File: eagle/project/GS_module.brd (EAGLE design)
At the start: 101.3 x 81.3 mm, 103 parts, among them IC1 LM358, Q2 MOSFET-PCHANNELFQP27P06, U1 V_REG_317SMD

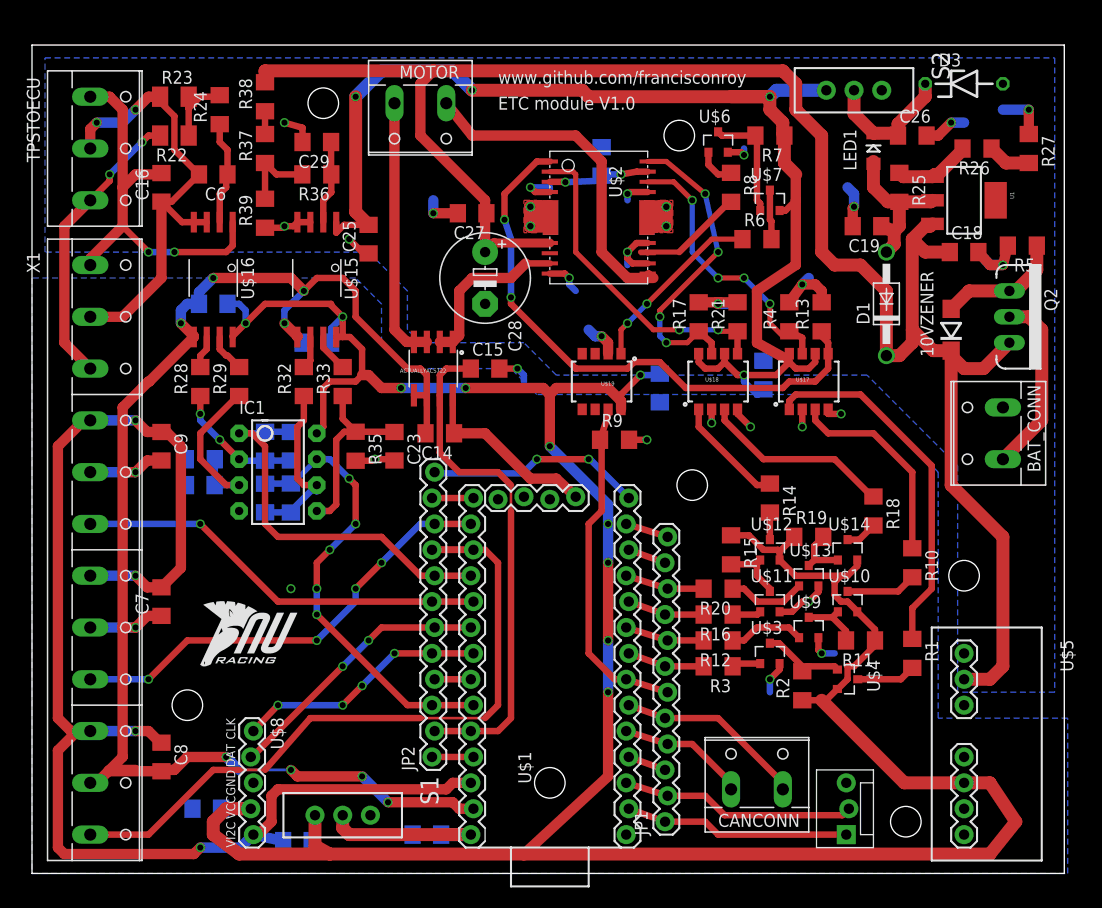
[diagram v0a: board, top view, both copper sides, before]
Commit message: finish version 1.0 of GS board
yay!
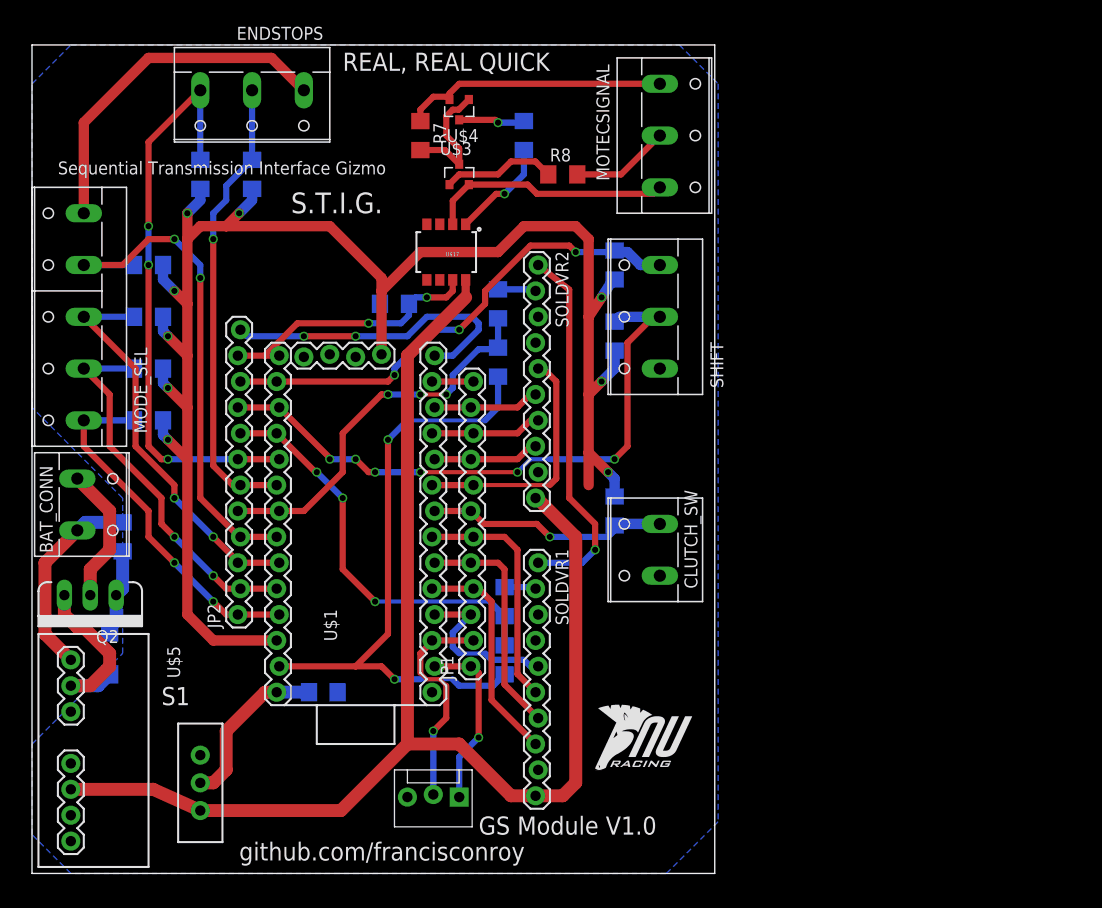
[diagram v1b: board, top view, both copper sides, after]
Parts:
- removed ACTUALLYACS722: ACS722, SparkFun-AnalogIC:SO08
- removed C10, C14, C8: 0.1 uF, rcl:C1206
- removed C13, C26, C3: 0.1uF, resistor:C1206
- removed C15, C20, C21, C22, C23: 1nF, rcl:C1206
- removed C16, C17, C18, C24, C25, C4, C5, C7, C9: 0.1uF, rcl:C1206
- removed C19, C27: 1uF, rcl:C1206
- removed C28: 47uF, rcl:E5-8,5
- removed C29, C6: 10n, rcl:C1206
- removed CANCONN, MOTOR: (no value), con-wago-508:W237-132
- removed D1: 1N4004, diode:DO41-10
- removed D3: 7.5V, diode:ZDIO-7.5
- removed IC1: LM358, SparkFun-AnalogIC:DIP08
- removed LED1: FUSE HERE, LilyPad-Wearables:LED-1206
- removed R19: 10k, resistor:R1206
- removed R20: 4.7k, resistor:R1206
- removed R21: 1k, resistor:R1206
- removed R22: 3k, rcl:M1206
- removed R23: 2k, rcl:M1206
- removed R24, R36: 39, rcl:R1206
- removed R25: 240, rcl:R1206
- removed R26: 680, rcl:R1206
- removed R27: 33, rcl:R1206
- removed R28, R29, R31, R32, R33, R35: 20k, rcl:R1206
- removed R30, R34: 40k, rcl:R1206
- removed R37: 56k, rcl:R1206
- removed R38: 4k7, rcl:R1206
- removed R39: 9k1, rcl:R1206
- removed S2: DIRTY 5V, SparkFun-Electromechanical:SWITCH-SPDT_KIT
- removed TPSTOECU: (no value), con-wago-508:W237-133
- removed U$10, U$12, U$14, U$7: PNP_TRAN, custom:SOT23-3
- removed U$11, U$13, U$6, U$9: NPN_TRAN, custom:SOT23-3
- removed U$15, U$16: ACPLC87BT, custom:SO8STRETCH
- removed U$18, U$19: OPTOISOLATOR-2SOIC8, SparkFun-DiscreteSemi:SO08-2
- removed U$20: (no value), custom:NURLOGO
- removed U$8: DISP_CONN, custom:DISP_CONN
- removed U1: V_REG_317SMD, SparkFun-PowerIC:SOT223
- removed X1: (no value), con-wago-508:W237-12P
- added CLUTCH_SW: (no value), con-wago-508:W237-132
- added ENDSTOPS, MOTECSIGNAL, SHIFT: (no value), con-wago-508:W237-133
- added MODE_SEL: (no value), con-wago-508:W237-5P
- added SOLDVR1, SOLDVR2: (no value), SparkFun-Connectors:1X10_LOCK
- R1: value 270 -> 27; device resistor:R1206 -> rcl:R1206
- R10, R14, R18: value 270 -> 10k; device resistor:R1206 -> rcl:R1206
- R11, R15: device resistor:R1206 -> rcl:R1206
- R12, R16: value 4.7k -> 10k; device resistor:R1206 -> rcl:R1206
- R13, R17: value 1k -> 10k; device resistor:R1206 -> rcl:R1206
- R2: value 10k -> 27; device resistor:R1206 -> rcl:R1206
- R3: value 4.7k -> 15; device resistor:R1206 -> rcl:R1206
- R4: value 1k -> 15; device resistor:R1206 -> rcl:R1206
- U$2: value TB6559FG -> (none); device custom:HSOP16-P-300-1.00 -> custom:NURLOGO
- moved Q2 94.2 mm to (5.71, 27.3), turned to 180 degrees
- moved R5 92.8 mm to (8.89, 33.0), flipped to the bottom, turned to 90 degrees
- moved BAT_CONN 89.8 mm to (5.08, 36.2), turned to 270 degrees
- moved 10VZENER 88.4 mm to (7.62, 21.6), flipped to the bottom
- moved U$5 87.6 mm to (3.81, 12.1)
- moved R12 68.3 mm to (16.5, 68.6), flipped to the bottom, turned to 270 degrees
- moved U$4 67.6 mm to (41.9, 74.9), turned to 180 degrees
- moved R14 65.1 mm to (11.4, 59.7), flipped to the bottom, turned to 180 degrees
- moved R15 61.6 mm to (11.4, 54.6), flipped to the bottom, turned to 180 degrees
- moved R16 60.9 mm to (11.4, 49.5), flipped to the bottom
- moved U$2 59.9 mm to (55.2, 10.2), turned to 0 degrees
- moved R13 57.6 mm to (21.6, 68.6), flipped to the bottom, turned to 270 degrees
- moved U$3 56.0 mm to (41.9, 68.6)
- moved R17 54.9 mm to (11.4, 44.5), flipped to the bottom, turned to 180 degrees
- moved R2 43.6 mm to (45.7, 50.2), flipped to the bottom
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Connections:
- removed net +5V/1: C13.1, C25.2, R7.1, S2.3, U$15.1, U$17.6, U$17.8, U$18.6, U$18.8, U$7.2
- removed net +5VCLEAN: C17.2, C24.2, C3.1, C4.2, IC1.8, R11.1, R15.1, R19.1, R2.1, S1.3, U$10.2, U$12.2, U$14.2, U$15.8, U$16.8, U$19.8, U$4.2, U$5.6, U$8.4
- removed net 5VOUT: C10.2, U$2.VREF, U$2.VREG
- removed net ECU5V: C16.2, TPSTOECU.1, U$16.1, X1.1
- removed net ECUSENSGND: C16.1, C6.2, R23.1, TPSTOECU.2, U$16.3, U$16.4, X1.2
- removed net ECUTPS: R22.2, TPSTOECU.3, X1.3
- removed net N$11: R8.1, U$6.1
- removed net N$12: R19.2, U$13.3, U$14.1
- removed net N$14: R18.1, U$18.3
- removed net N$15: C26.1, D3.C, LED1.C, S2.2
- removed net N$16: R37.2, R38.1
- removed net N$17: C19.1, D1.A, LED1.A, R25.2, U1.2
- removed net N$18: R11.2, U$10.1, U$9.3
- removed net N$19: MOTOR.1, U$2.OUT2
- removed net N$20: ACTUALLYACS722.1, ACTUALLYACS722.2, U$2.OUT1
- removed net N$21: R10.1, U$17.3
- removed net N$22: R10.2, U$10.3
- removed net N$23: R12.1, U$9.1
- removed net N$25: R15.2, U$11.3, U$12.1
- removed net N$26: R14.1, U$18.1
- removed net N$27: R14.2, U$12.3
- removed net N$28: R16.1, U$11.1
- removed net N$29: R17.1, U$18.7, U$2.IN2
- removed net N$30: R18.2, U$14.3
- removed net N$31: R20.1, U$13.1
- removed net N$32: R8.2, U$2.ALERT
- removed net N$33: R21.1, U$18.5, U$2.SB
- removed net N$34: ACTUALLYACS722.3, ACTUALLYACS722.4, MOTOR.2
- removed net N$35: C6.1, R24.1, U$16.2
- removed net N$36: R22.1, R23.2, R24.2
- removed net N$37: R26.1, R27.2
- removed net N$38: R25.1, R26.2, U1.1
- removed net N$39: R36.2, R37.1, R39.2
- removed net N$40: C23.1, IC1.5, R33.1, R35.1
- removed net N$41: C22.2, IC1.6, R32.1, R34.2
- removed net N$42: R32.2, U$15.6
- removed net N$43: R13.1, U$17.5, U$2.IN1
- removed net N$44: R29.2, U$16.7
- removed net N$45: C21.1, IC1.3, R29.1, R31.1
- removed net N$46: C20.2, IC1.2, R28.1, R30.2
- removed net N$47: R28.2, U$16.6
- removed net N$48: C29.1, R36.1, U$15.2
- removed net N$52: R33.2, U$15.7
- new net +5V: S1.3, SOLDVR1.10, SOLDVR2.10, U$17.8, U$5.6
- new net +5V/4: MOTECSIGNAL.1, R7.1, U$4.2
- new net GND4: MOTECSIGNAL.3, U$17.2, U$3.2
- net +12V: no longer C18.1, C27.1, C28.+, D1.C, R38.2, U$2.VCC, U1.3
- net +3V3: now also R10.2, R11.2, R12.2, R13.2, R14.2, R15.2, R16.2, R17.2, R18.2; no longer ACTUALLYACS722.8, C14.1, C5.2, C7.2, C8.1, C9.1, U$8.5, X1.10, X1.4, X1.7
- net AGND: now also R1.1, R2.1; no longer ACTUALLYACS722.5, ACTUALLYACS722.6, C14.2, C17.1, C24.1, C7.1, C8.2, C9.2, U$15.5, U$16.5, X1.11, X1.5, X1.8
- net GND: now also CLUTCH_SW.1, ENDSTOPS.1, MODE_SEL.5, SHIFT.1, SOLDVR1.9, SOLDVR2.9; no longer C15.2, C21.2, C23.2, C3.2, C4.1, C5.1, IC1.4, R31.2, R35.2, U$11.2, U$13.2, U$17.2, U$17.4, U$18.2, U$18.4, U$3.2, U$8.3, U$9.2
- net GNDI: no longer C10.1, C13.2, C18.2, C19.2, C25.1, C26.2, C27.2, C28.-, C29.2, D3.A, R13.2, R17.2, R21.2, R27.1, R39.1, R4.2, S2.1, U$15.3, U$15.4, U$19.2, U$2.FIN, U$2.FIN2, U$2.P$20, U$2.P$4, U$2.P-GND, U$2.RSA, U$2.S-GND, U$2.S-GND2, U$2.S-GND3, U$6.2
- net N$1: now also R7.2; no longer R2.2
- net N$10: now also SOLDVR1.1, SOLDVR2.1; no longer R6.2, U$7.3
- net N$3: now also R3.2, SOLDVR1.2; no longer R1.1, U$17.1
- net N$4: now also R6.1, U$17.1; no longer R1.2, U$4.3
- net N$5: now also R4.2, SOLDVR2.2; no longer R3.1, U$3.1
- net N$6: now also R6.2, U$4.3; no longer R7.2, U$6.3, U$7.1
- net N$8: now also R8.1, U$3.1; no longer R4.1, U$17.7, U$2.PWM
- net N$9: now also MOTECSIGNAL.2, R8.2; no longer R6.1, U$19.1
- net P10: now also SOLDVR2.6
- net P13: now also R9.1, U$17.7
- net P14: now also R10.1, SHIFT.3; no longer X1.9
- net P15: now also R11.1, SHIFT.2; no longer X1.12
- net P16: now also R1.2, R3.1; no longer C20.1, IC1.1, R30.1
- net P17: now also ENDSTOPS.3, R12.1; no longer X1.6
- net P18: now also ENDSTOPS.2, R13.1; no longer U$8.2
- net P19: now also R2.2, R4.1; no longer U$8.1
- net P2: now also SOLDVR1.5
- net P20: now also MODE_SEL.4, R14.1
- net P21: now also MODE_SEL.3, R15.1; no longer C22.1, IC1.7, R34.1
- net P22: now also MODE_SEL.2, R16.1; no longer ACTUALLYACS722.7, C15.1
- net P23: now also MODE_SEL.1, R17.1
- net P3: now also SOLDVR1.8; no longer CANCONN.1
- net P4: now also SOLDVR1.7; no longer CANCONN.2
- net P5: now also SOLDVR1.6; no longer R9.1, U$19.7
- net P6: now also CLUTCH_SW.2, R18.1; no longer R3.2
- net P7: now also SOLDVR2.5; no longer R12.2
- net P8: now also SOLDVR2.8; no longer R16.2
- net P9: now also SOLDVR2.7; no longer R20.2
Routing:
- net +5VCLEAN: track 276.3 -> 0.00 mm, vias 10 -> 0
- net +12V: track 183.3 -> 18.1 mm
- net +5V: track 0.00 -> 132.9 mm
- net +5V/1: track 123.2 -> 0.00 mm, vias 4 -> 0
- net AGND: track 158.1 -> 62.0 mm, vias 10 -> 2
- net GNDI: track 96.0 -> 19.8 mm, vias 20 -> 0
- net N$43: track 56.4 -> 0.00 mm, vias 2 -> 0
- net P20: track 3.56 -> 50.4 mm, vias 0 -> 2
- net ECUSENSGND: track 45.4 -> 0.00 mm, vias 2 -> 0
- net ECU5V: track 39.1 -> 0.00 mm, vias 2 -> 0
- net N$19: track 33.6 -> 0.00 mm
- net N$3: track 35.7 -> 3.11 mm
- net N$10: track 4.87 -> 36.6 mm, vias 0 -> 1
- net N$33: track 31.6 -> 0.00 mm, vias 2 -> 0
- net P23: track 4.06 -> 35.0 mm, vias 0 -> 2
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- removed copper zone on layer 1, net GNDI
- removed copper zone on layer 16, net GNDI
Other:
- board size 101.3 x 81.3 mm -> 67 x 81.3 mm
- board text added: "GS Module V1.0"
- board text added: "REAL, REAL QUICK"
- board text added: "S.T.I.G."
- board text added: "Sequential Transmission Interface Gizmo"
- board text added: "github.com/francisconroy"
- board text removed: "ETC module V1.0"
- board text removed: "www.github.com/francisconroy"
